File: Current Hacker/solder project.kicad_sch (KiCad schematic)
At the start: 12 parts, among them J1 Conn_01x01_Pin, M1 Motor_DC, Q1 2N3904, Q2 2N3904, Q3 2N3904, SW1 SW_Push

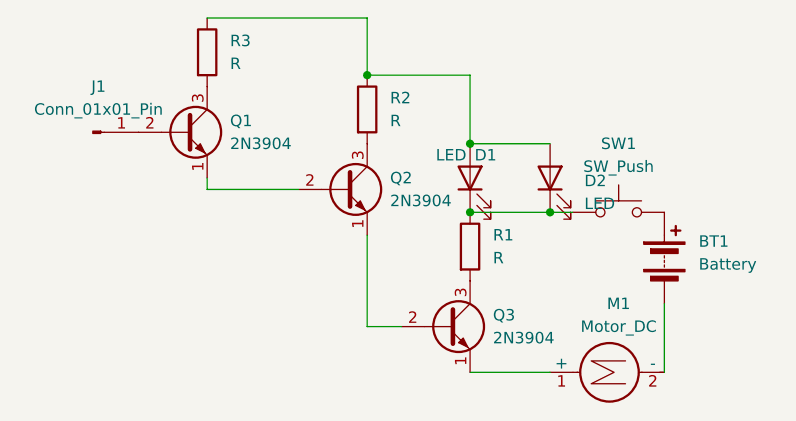
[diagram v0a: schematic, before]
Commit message: Add files via upload
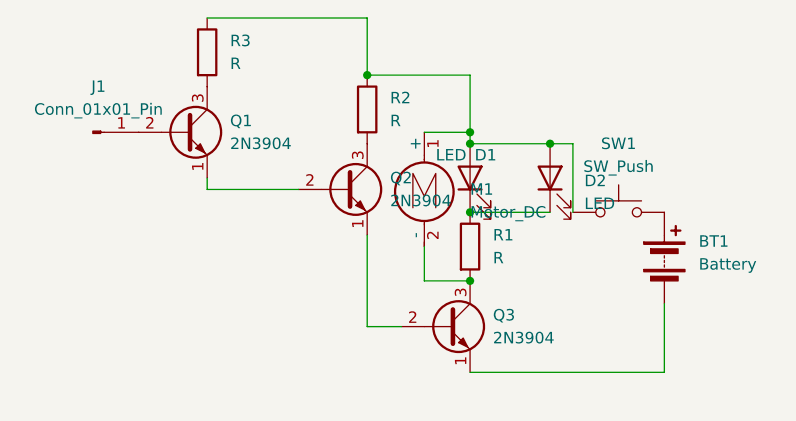
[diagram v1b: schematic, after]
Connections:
- net at D1.1 (K), D2.1 (K), R1.1: no longer SW1.1
- net at Q3.3 (C), R1.2: now also M1.2 (-)
- net at Q3.1 (E): now also BT1.2 (-); no longer M1.1 (+)
- net at D1.2 (A), D2.2 (A), R2.1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: now also M1.1 (+), SW1.1
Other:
- moved on the sheet: M1
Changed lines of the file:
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@@
 	)
 	(junction
-		(at 214.63 68.58)
+		(at 214.63 60.96)
+		(diameter 0)
+		(color 0 0 0 0)
+	)
+	(junction
+		(at 205.74 76.2)
+		(diameter 0)
+		(color 0 0 0 0)
+	)
+	(junction
+		(at 205.74 59.69)
 		(diameter 0)
 		(color 0 0 0 0)
@@
 	(wire
 		(pts
-			(xy 214.63 68.58) (xy 217.17 68.58)
-		)
-		(stroke
-			(width 0)
-			(type default)
-		)
-	)
-	(wire
-		(pts
 			(xy 176.53 66.04) (xy 186.69 66.04)
 		)
@@
 	(wire
 		(pts
-			(xy 205.74 53.34) (xy 205.74 60.96)
-		)
-		(stroke
-			(width 0)
-			(type default)
-		)
-	)
-	(wire
-		(pts
-			(xy 205.74 86.36) (xy 214.63 86.36)
+			(xy 200.66 72.39) (xy 200.66 76.2)
+		)
+		(stroke
+			(width 0)
+			(type default)
+		)
+	)
+	(wire
+		(pts
+			(xy 205.74 53.34) (xy 205.74 59.69)
+		)
+		(stroke
+			(width 0)
+			(type default)
+		)
+	)
+	(wire
+		(pts
+			(xy 205.74 86.36) (xy 227.33 86.36)
 		)
 		(stroke
@@
 	(wire
 		(pts
+			(xy 200.66 76.2) (xy 205.74 76.2)
+		)
+		(stroke
+			(width 0)
+			(type default)
+		)
+	)
+	(wire
+		(pts
+			(xy 205.74 59.69) (xy 205.74 60.96)
+		)
+		(stroke
+			(width 0)
+			(type default)
+		)
+	)
+	(wire
+		(pts
 			(xy 176.53 66.04) (xy 176.53 64.77)
 		)
@@
 	(wire
 		(pts
+			(xy 217.17 68.58) (xy 217.17 60.96)
+		)
+		(stroke
+			(width 0)
+			(type default)
+		)
+	)
+	(wire
+		(pts
 			(xy 205.74 60.96) (xy 214.63 60.96)
 		)
@@
 	(wire
 		(pts
+			(xy 217.17 60.96) (xy 214.63 60.96)
+		)
+		(stroke
+			(width 0)
+			(type default)
+		)
+	)
+	(wire
+		(pts
 			(xy 227.33 86.36) (xy 227.33 78.74)
+		)
+		(stroke
+			(width 0)
+			(type default)
+		)
+	)
+	(wire
+		(pts
+			(xy 200.66 59.69) (xy 205.74 59.69)
 		)
 		(stroke
@@
 	(symbol
 		(lib_id "Motor:Motor_DC")
-		(at 219.71 86.36 90)
+		(at 200.66 64.77 0)
 		(unit 1)
 		(exclude_from_sim no)
@@
 		(fields_autoplaced yes)
 		(property "Reference" "M1"
-			(at 222.25 78.74 90)
-			(effects
-				(font
-					(size 1.27 1.27)
-				)
+			(at 205.74 66.0399 0)
+			(effects
+				(font
+					(size 1.27 1.27)
+				)
+				(justify left)
 			)
 		)
 		(property "Value" "Motor_DC"
-			(at 222.25 81.28 90)
-			(effects
-				(font
-					(size 1.27 1.27)
-				)
+			(at 205.74 68.5799 0)
+			(effects
+				(font
+					(size 1.27 1.27)
+				)
+				(justify left)
 			)
 		)
 		(property "Footprint" "Connector_PinHeader_2.54mm:PinHeader_1x02_P2.54mm_Vertical"
-			(at 221.996 86.36 0)
+			(at 200.66 67.056 0)
 			(effects
 				(font
@@
 		)
 		(property "Datasheet" "~"
-			(at 221.996 86.36 0)
+			(at 200.66 67.056 0)
 			(effects
 				(font
@@
 		)
 		(property "Description" "DC Motor"
-			(at 219.71 86.36 0)
+			(at 200.66 64.77 0)
 			(effects
 				(font
@@
 		)
 		(property "Sim.Device" ""
-			(at 219.71 86.36 0)
-			(effects
-				(font
+			(at 200.66 64.77 0)
+			(effects
+				(font
